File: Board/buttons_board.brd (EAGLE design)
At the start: 35 x 27.4 mm, 5 parts, among them U1 TEM-HUM-AM2302(4P-25.0X15.0MM)

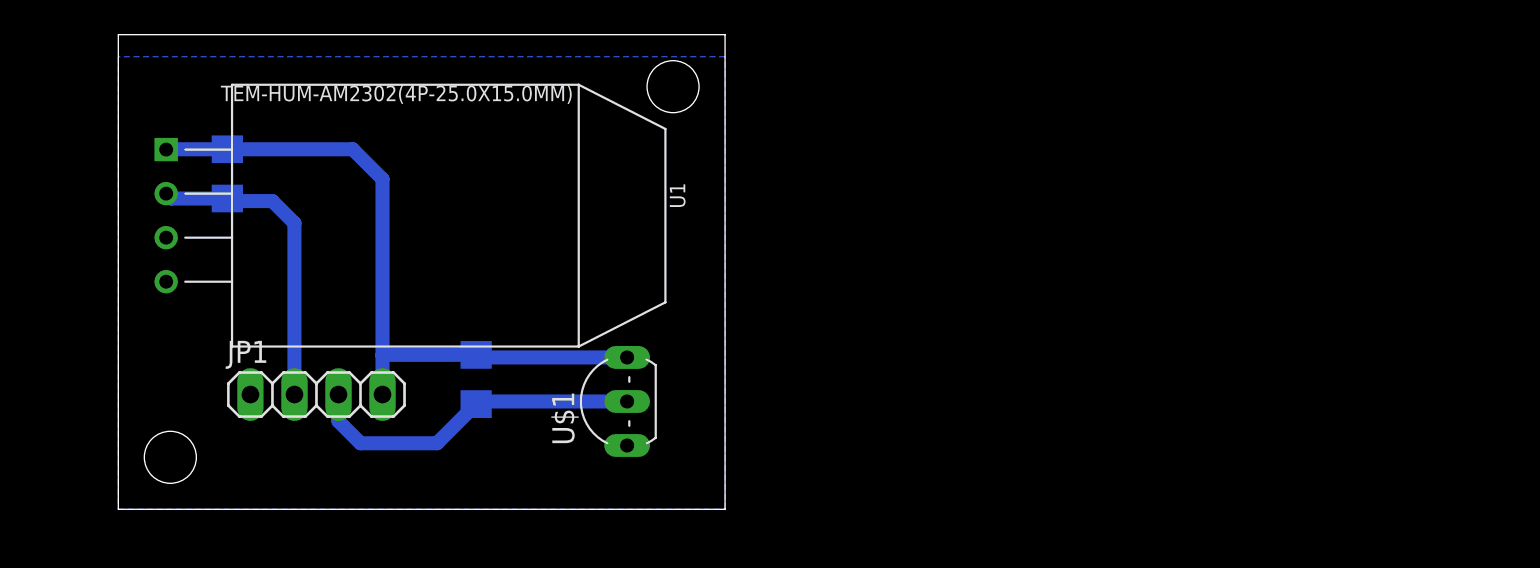
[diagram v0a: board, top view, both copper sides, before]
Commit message: Update
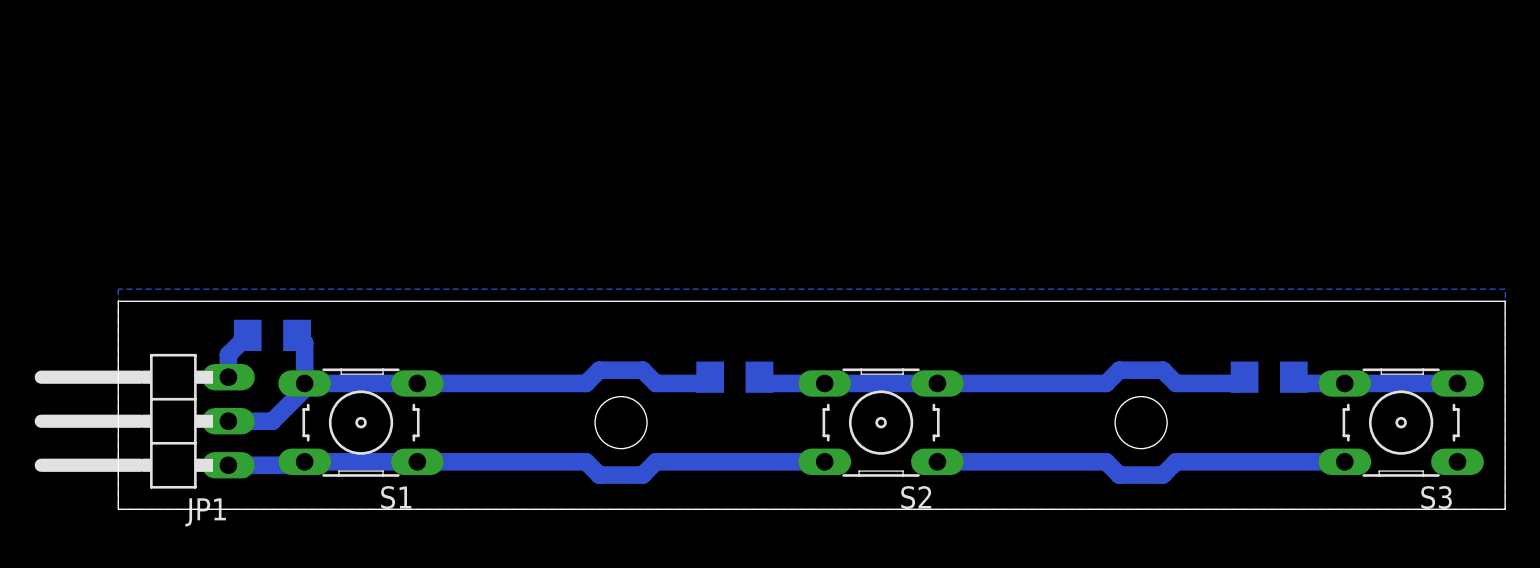
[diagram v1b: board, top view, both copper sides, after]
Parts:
- removed U$1: DS18B20, DS18B20_PAR:TO92-
- removed U1: TEM-HUM-AM2302(4P-25.0X15.0MM), TEM-HUM-AM2302_4P-25.0X15.0MM_:SNR4-2.54-25.0X15.0X7.0MM
- added R3: 10k, rcl:R1206
- added S1, S2, S3: (no value), switch-omron:B3F-10XX
- JP1: device pinhead:1X04 -> pinhead:1X03/90
- R1, R2: value (none) -> 10k
- moved R1 45.8 mm to (66.4, 7.62), turned to 180 degrees
- moved R2 31.5 mm to (35.6, 7.62), turned to 180 degrees
- moved JP1 9.02 mm to (2.54, 5.08), turned to 90 degrees
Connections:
- new net N$3: R1.2, S3.3, S3.4
- net +3V3: now also JP1.1, S1.1, S1.2, S2.1, S2.2, S3.1, S3.2; no longer JP1.4, R1.2, R2.2, U$1.1, U1.P$1
- net GND: now also JP1.3, R3.1; no longer JP1.1, U$1.3, U1.P$4
- net N$1: now also R3.2, S1.3, S1.4; no longer U1.P$2
- net N$2: now also R2.2, S2.3, S2.4; no longer JP1.3, U$1.2
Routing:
- net +3V3: track 40.2 -> 59.2 mm
- net N$1: track 18.0 -> 32.7 mm
- net N$3: track 0.00 -> 9.59 mm
- net N$2: track 19.7 -> 28.9 mm
- net GND: track 0.00 -> 2.88 mm
- added copper zone on layer 16, net POLYGON
- removed copper zone on layer 16, net GND
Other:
- board size 35 x 27.4 mm -> 80 x 12 mm
